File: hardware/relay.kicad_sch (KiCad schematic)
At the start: 4 parts, among them K1 G5Q-1, U4 TCMT1100

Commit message: added historical scripts and new revisions
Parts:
- K1: TC_DATAsheet (none) -> https://www.omron.com/ecb/products/pdf/en-g5q.pdf
- U4: TC_DATAsheet (none) -> http://www.vishay.com/docs/83510/tcmt1100.pdf
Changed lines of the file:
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@@
 			)
 		)
-		(property "Datasheet" "http://www.vishay.com/docs/83510/tcmt1100.pdf"
+		(property "TC_DATAsheet" "http://www.vishay.com/docs/83510/tcmt1100.pdf"
 			(at 137.16 90.17 0)
 			(effects
@@
 			)
 		)
-		(property "Datasheet" "~"
+		(property "TC_DATAsheet" "~"
 			(at 138.43 69.85 0)
 			(effects
@@
 			)
 		)
-		(property "Datasheet" ""
+		(property "TC_DATAsheet" ""
 			(at 119.38 86.36 90)
 			(effects
@@
 			)
 		)
-		(property "Datasheet" "https://www.omron.com/ecb/products/pdf/en-g5q.pdf"
+		(property "TC_DATAsheet" "https://www.omron.com/ecb/products/pdf/en-g5q.pdf"
 			(at 156.21 68.58 0)
 			(effects

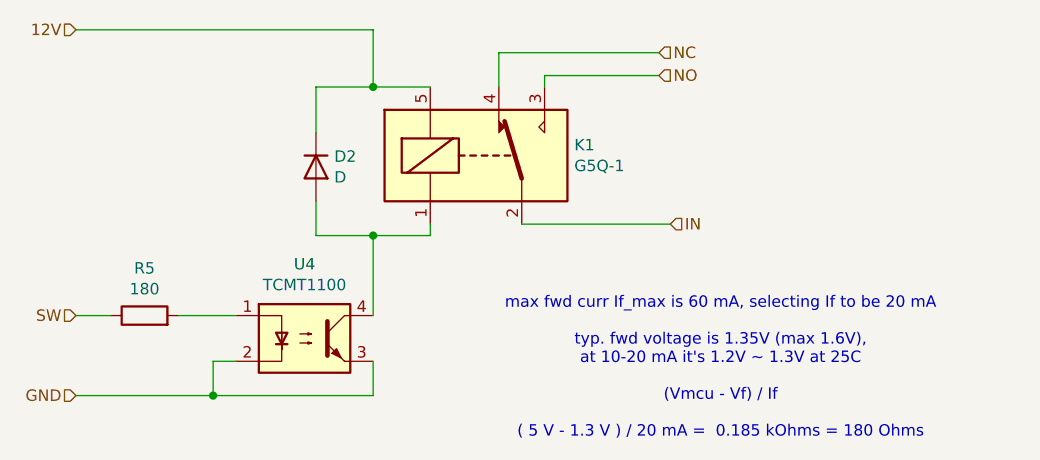
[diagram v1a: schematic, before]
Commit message: review and revise for current template and kmlib; still needs updating
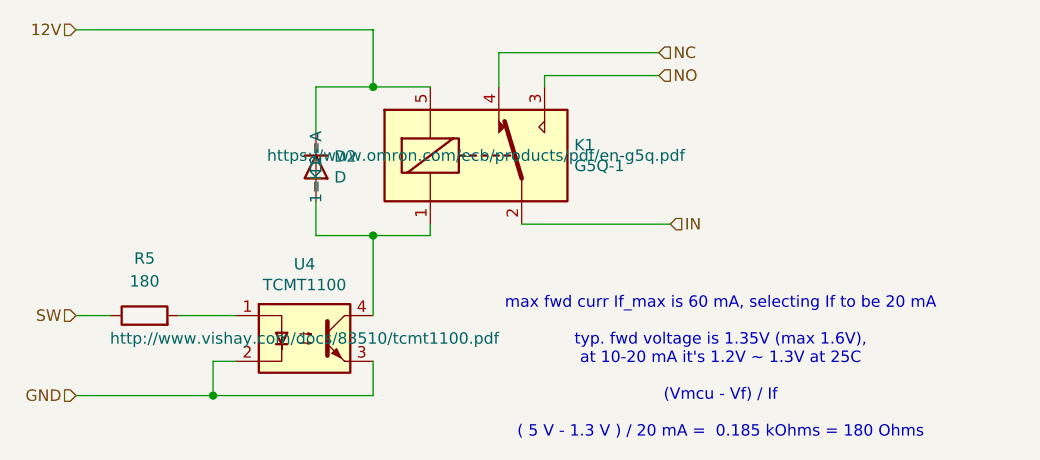
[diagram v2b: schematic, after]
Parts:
- removed R5: 180, Resistor_SMD:R_1206_3216Metric_Pad1.30x1.75mm_HandSolder, symbol BREAD_Slice-rescue:R-OCI_UPL_1_Resistors
- added R5: 180, Resistor_SMD:R_1206_3216Metric_Pad1.30x1.75mm_HandSolder, symbol Device:R
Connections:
- net SW: now also R5.1
- net at U4.1: now also R5.2
